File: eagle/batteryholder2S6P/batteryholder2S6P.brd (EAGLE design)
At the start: 185.4 x 89.7 mm, 10 parts, among them J3 POWER_JACKPTH_BREAD

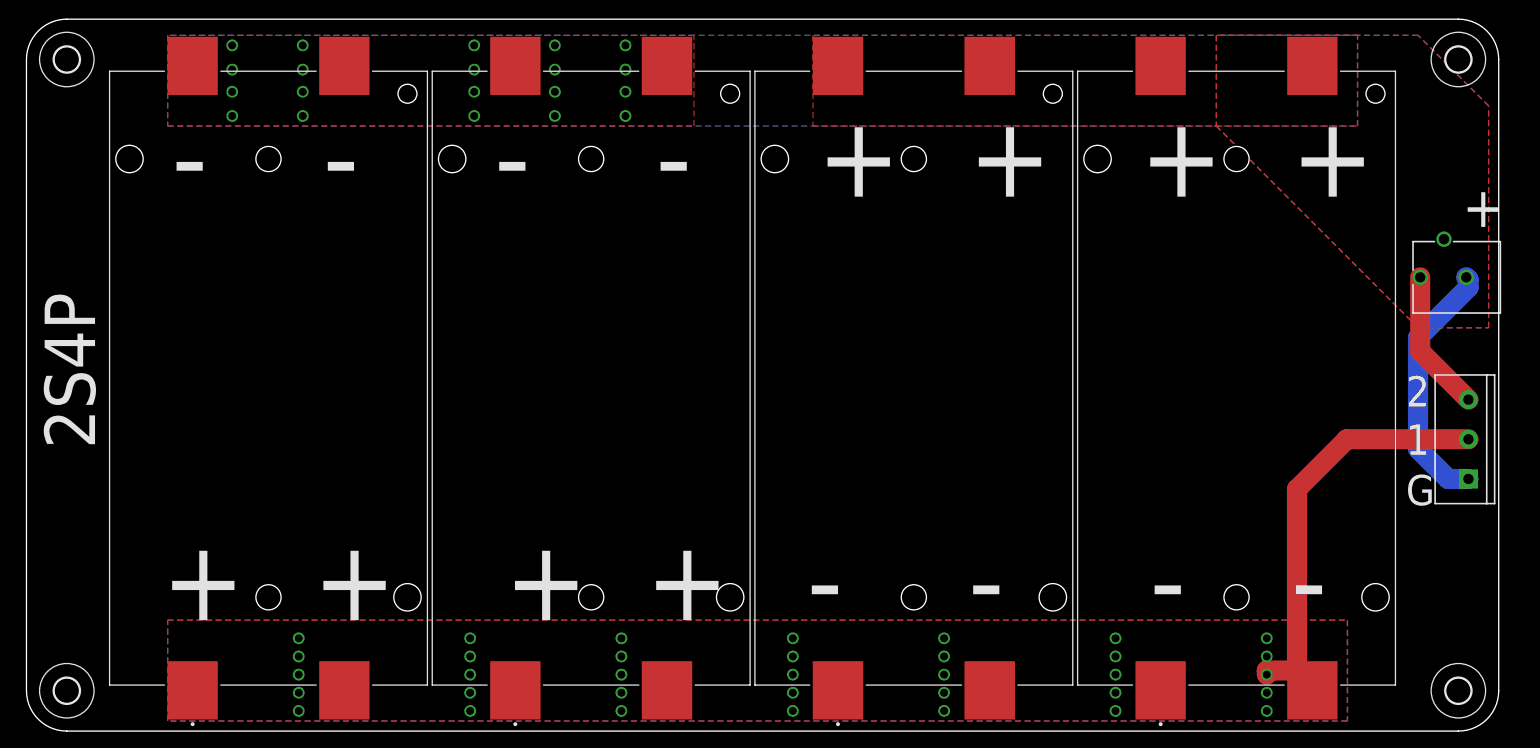
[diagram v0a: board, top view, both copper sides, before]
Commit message: new PCB files (batteryholder, templog2, ...)
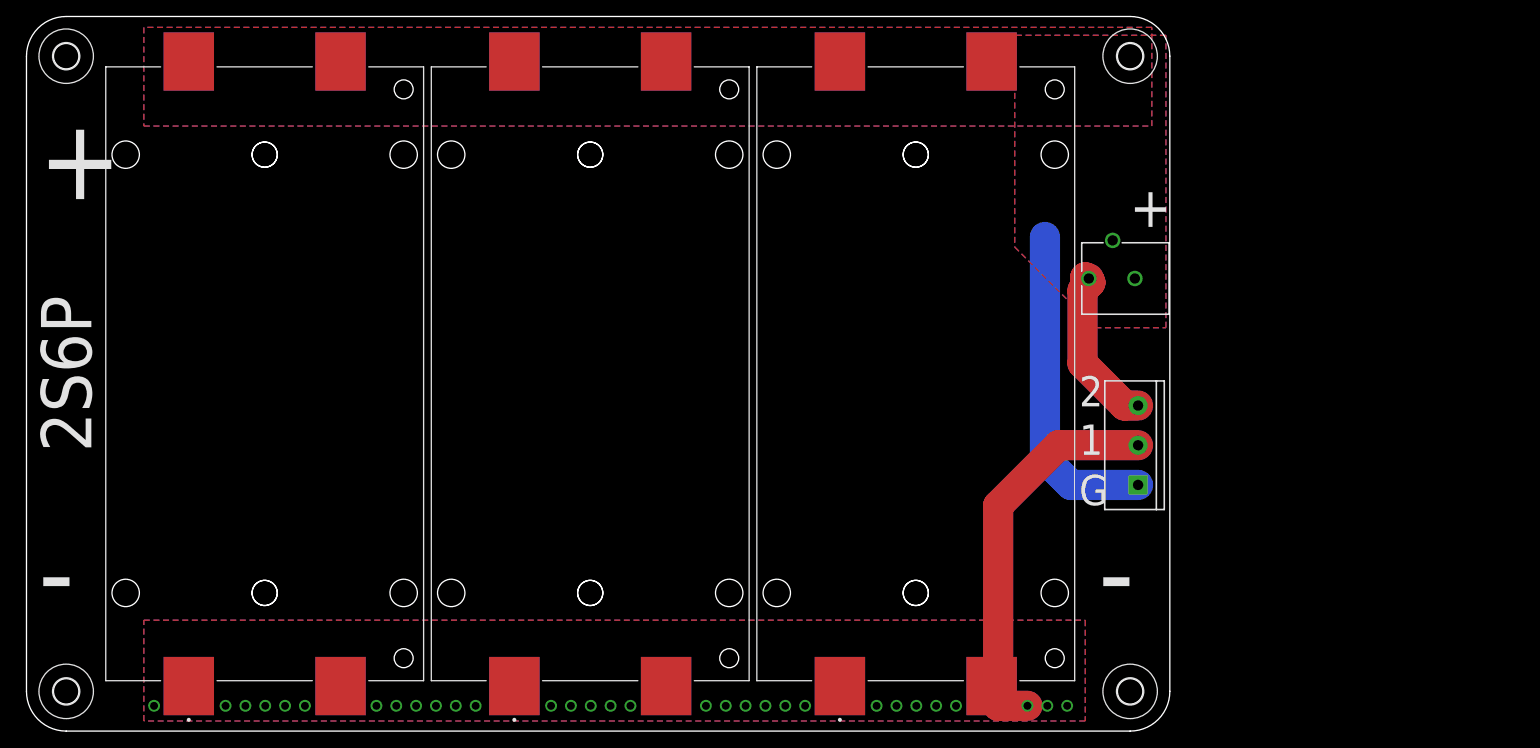
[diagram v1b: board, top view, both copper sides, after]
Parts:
- removed BT4: KEYSTONE_1048KEYSTONE_1048_0_0, Keystone - 1048:KEYSTONE_1048_0
- added BT5, BT6, BT7: KEYSTONE_1048KEYSTONE_1048_0_0, Keystone - 1048:KEYSTONE_1048_0
- moved J3 41.7 mm to (147.5, 57.0)
- moved J1 41.6 mm to (140.0, 31.0)
- moved H3 41.3 mm to (139.0, 85.0)
- moved H4 41.3 mm to (139.0, 5.00)
- moved BT1 0.73 mm to (30.0, 45.0)
- moved BT3 0.60 mm to (112.0, 45.0)
- moved BT2 0.56 mm to (71.0, 45.0)
- moved H1 0.43 mm to (5.00, 85.0)
- moved H2 0.11 mm to (5.00, 5.00)
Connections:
- net BOTTOM_MINUS: now also BT5.1, BT5.3, BT6.1, BT6.3, BT7.1, BT7.3; no longer BT1.2, BT1.4, BT2.2, BT2.4
- net TOP_MINUS: now also BT5.2, BT5.4, BT6.2, BT6.4, BT7.2, BT7.4; no longer BT4.1, BT4.3
- net TOP_PLUS: now also BT1.2, BT1.4, BT2.2, BT2.4; no longer BT4.2, BT4.4
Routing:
- net BOTTOM_MINUS: track 32.3 -> 41.0 mm, vias 20 -> 0
- net TOP_PLUS: track 17.9 -> 21.2 mm
- net TOP_MINUS: track 51.4 -> 49.7 mm, vias 35 -> 31
- removed copper zone on layer 1, net BOTTOM_MINUS
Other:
- board size 185.4 x 89.7 mm -> 144 x 90 mm
- board text added: "2S6P"
- board text removed: "2S4P"
